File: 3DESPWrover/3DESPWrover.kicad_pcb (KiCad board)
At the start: 2 copper layers, 40 x 40 mm, 21 parts, among them J1 Conn_01x05_Male, J2 Conn_01x03_Female, J3 Conn_02x03_Odd_Even, J4 Conn_02x07_Odd_Even, SW1 SW_Push, SW2 SW_Push, U1 ESP32-S2-WROVER

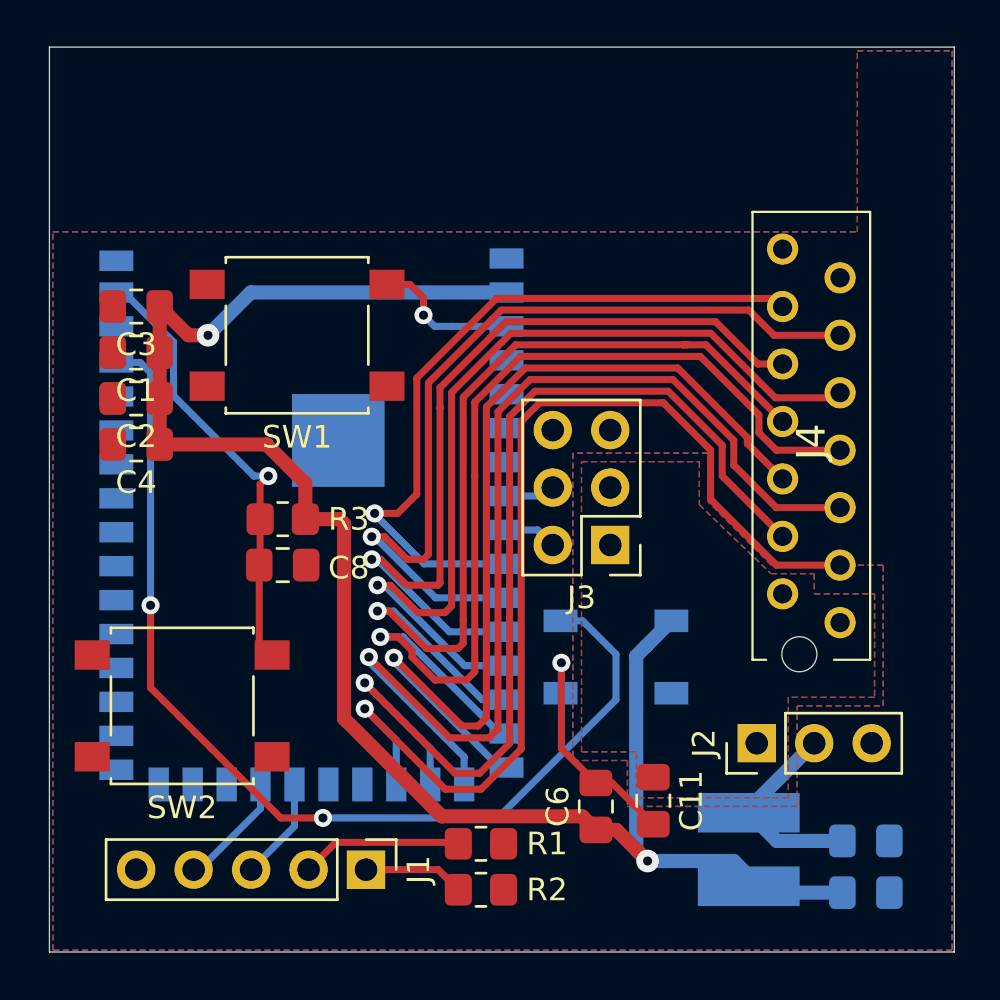
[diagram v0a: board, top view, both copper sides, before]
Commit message: Cleared Andres comments
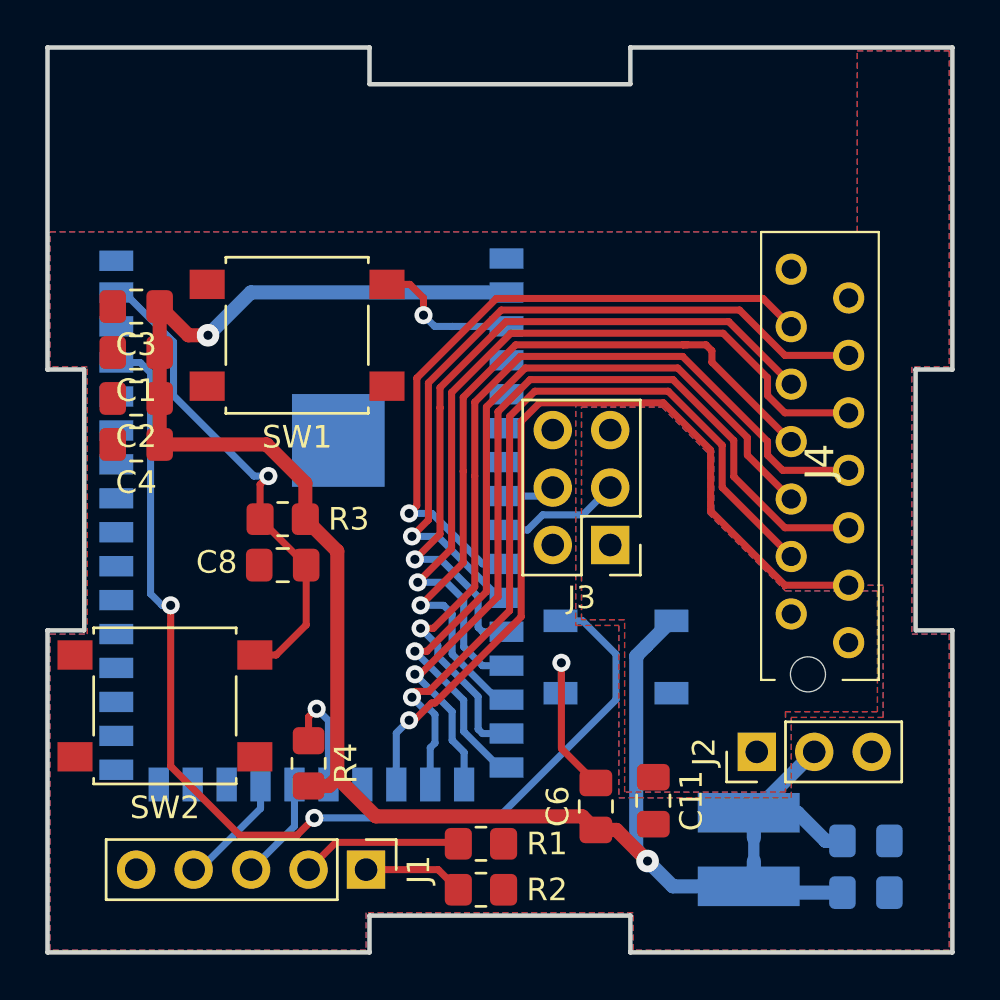
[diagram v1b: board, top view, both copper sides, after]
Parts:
- added NT1: Net-Tie_2, NetTie:NetTie-2_SMD_Pad0.5mm, B.Cu at (231.1, 85.5)
- added R4: 10k, Resistor_SMD:R_0805_2012Metric_Pad1.20x1.40mm_HandSolder, F.Cu at (211.5, 81.7)
- moved J4 0.97 mm to (232.8, 59.8)
- moved SW2 0.76 mm to (205.1, 79.1)
- moved J2 0.38 mm to (231.3, 81.2)
- turned C8 to 180 degrees
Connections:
- J3 pad 2: /D6 -> GND
- J3 pad 3: /Vin -> /D6
- J3 pad 5: GND -> /Vin
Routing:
- net /D14: track 47.4 -> 38.8 mm
- net /D15: track 44.7 -> 36.1 mm
- net /D16: track 46.2 -> 38.3 mm
- net /D13: track 42.3 -> 36.5 mm
- net /D12: track 43.7 -> 38.3 mm
- net /D11: track 39.4 -> 34.3 mm
- net /AD1: track 0.00 -> 5.12 mm, vias 0 -> 1
- net /D8: track 37.7 -> 33.1 mm
- net /D9: track 36.6 -> 32.1 mm
- net /D10: track 40.0 -> 36.2 mm
- net +3V3: track 79.1 -> 82.7 mm
- net GND: track 10.6 -> 7.31 mm
- net /D6: track 2.32 -> 5.36 mm
- net /NEOPIX: track 46.2 -> 48.5 mm
- net /RESET: track 19.8 -> 21.9 mm
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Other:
- outline, holes or cut-outs redrawn
